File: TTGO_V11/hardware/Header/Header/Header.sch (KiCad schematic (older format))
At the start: 1 part

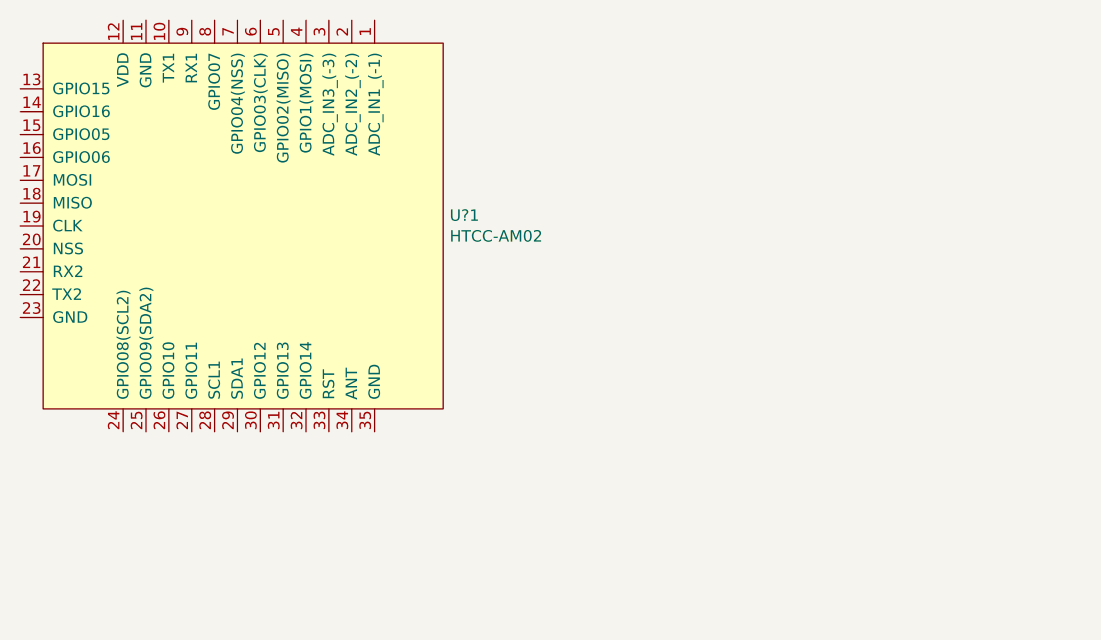
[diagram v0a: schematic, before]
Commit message: design changes
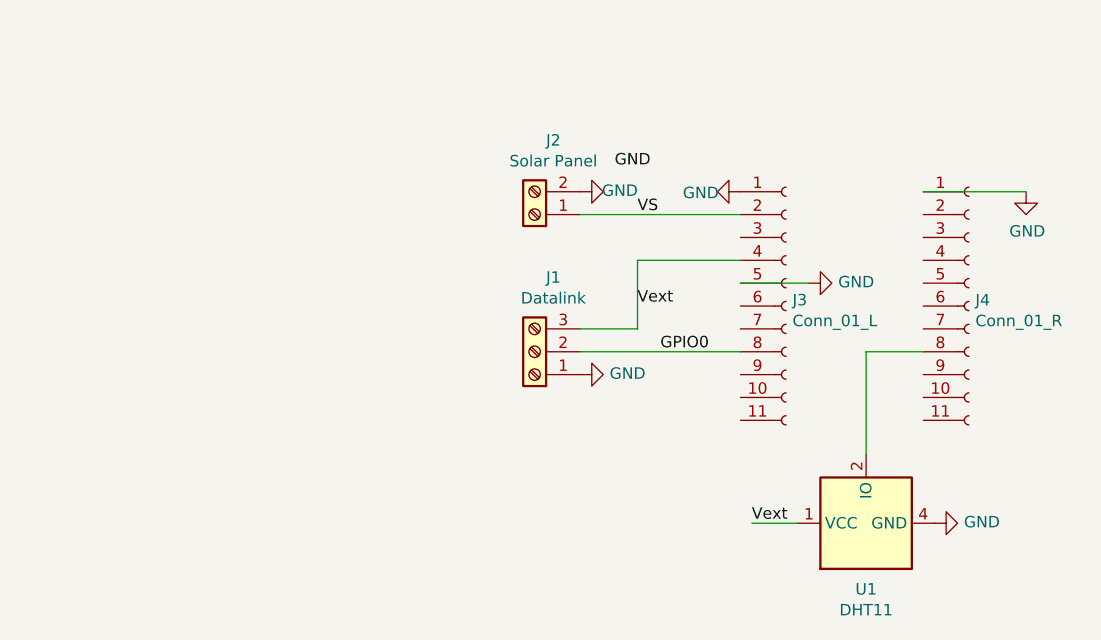
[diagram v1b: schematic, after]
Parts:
- removed U?1: HTCC-AM02, symbol htcc:HTCC-AM02
- added J1: Datalink, TerminalBlock_MetzConnect:TerminalBlock_MetzConnect_Type101_RT01603HBWC_1x03_P5.08mm_Horizontal, symbol Connector:Screw_Terminal_01x03
- added J2: Solar Panel, TerminalBlock_MetzConnect:TerminalBlock_MetzConnect_Type101_RT01602HBWC_1x02_P5.08mm_Horizontal, symbol Connector:Screw_Terminal_01x02
- added J3: Conn_01_L, Connector_PinHeader_2.54mm:PinHeader_1x11_P2.54mm_Vertical, symbol Connector:Conn_01x11_Female
- added J4: Conn_01_R, Connector_PinHeader_2.54mm:PinHeader_1x11_P2.54mm_Vertical, symbol Connector:Conn_01x11_Female
- added U1: DHT11, Sensor:Aosong_DHT11_5.5x12.0_P2.54mm, symbol Sensor:DHT11
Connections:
- new net: J4.8 (Pin_8), U1.2 (IO)
- new net GND: J1.1 (Pin_1), J2.2 (Pin_2), J3.1 (Pin_1), J3.5 (Pin_5), J4.1 (Pin_1), U1.4 (GND)
- new net GPIO0: J1.2 (Pin_2), J3.8 (Pin_8)
- new net VS: J2.1 (Pin_1), J3.2 (Pin_2)
- new net Vext: J1.3 (Pin_3), J3.4 (Pin_4), U1.1 (VCC)
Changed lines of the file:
@@
 $EndDescr
 $Comp
-L htcc:HTCC-AM02 U?1
-U 1 1 608BC1DC
-P 5750 3550
-F 0 "U?1" H 6678 3596 50  0000 L CNN
-F 1 "HTCC-AM02" H 6678 3505 50  0000 L CNN
-F 2 "" H 5800 4150 50  0001 C CNN
-F 3 "" H 5800 4150 50  0001 C CNN
-	1    5750 3550
+L Connector:Screw_Terminal_01x03 J1
+U 1 1 608CA66F
+P 7050 4100
+F 0 "J1" H 6968 3775 50  0000 C CNN
+F 1 "Datalink" H 6968 3866 50  0000 C CNN
+F 2 "TerminalBlock_MetzConnect:TerminalBlock_MetzConnect_Type101_RT01603HBWC_1x03_P5.08mm_Horizontal" H 7050 4100 50  0001 C CNN
+F 3 "~" H 7050 4100 50  0001 C CNN
+	1    7050 4100
+	-1   0    0    1
+$EndComp
+$Comp
+L Connector:Screw_Terminal_01x02 J2
+U 1 1 608CAD5D
+P 7050 3500
+F 0 "J2" H 6968 3175 50  0000 C CNN
+F 1 "Solar Panel" H 6968 3266 50  0000 C CNN
+F 2 "TerminalBlock_MetzConnect:TerminalBlock_MetzConnect_Type101_RT01602HBWC_1x02_P5.08mm_Horizontal" H 7050 3500 50  0001 C CNN
+F 3 "~" H 7050 3500 50  0001 C CNN
+	1    7050 3500
+	-1   0    0    1
+$EndComp
+$Comp
+L Connector:Conn_01x11_Female J3
+U 1 1 608CB784
+P 8150 3900
+F 0 "J3" H 8178 3926 50  0000 L CNN
+F 1 "Conn_01_L" H 8178 3835 50  0000 L CNN
+F 2 "Connector_PinHeader_2.54mm:PinHeader_1x11_P2.54mm_Vertical" H 8150 3900 50  0001 C CNN
+F 3 "~" H 8150 3900 50  0001 C CNN
+	1    8150 3900
 	1    0    0    -1
 $EndComp
+$Comp
+L Connector:Conn_01x11_Female J4
+U 1 1 608D10F0
+P 8950 3900
+F 0 "J4" H 8978 3926 50  0000 L CNN
+F 1 "Conn_01_R" H 8978 3835 50  0000 L CNN
+F 2 "Connector_PinHeader_2.54mm:PinHeader_1x11_P2.54mm_Vertical" H 8950 3900 50  0001 C CNN
+F 3 "~" H 8950 3900 50  0001 C CNN
+	1    8950 3900
+	1    0    0    -1
+$EndComp
+$Comp
+L power:GND #PWR0101
+U 1 1 608D6208
+P 7950 3400
+F 0 "#PWR0101" H 7950 3150 50  0001 C CNN
+F 1 "GND" V 7955 3227 50  0000 C CNN
+F 2 "" H 7950 3400 50  0001 C CNN
+F 3 "" H 7950 3400 50  0001 C CNN
+	1    7950 3400
+	0    1    1    0
+$EndComp
+Wire Wire Line
+	7950 3500 7250 3500
+Text Label 7500 3500 0    50   ~ 0
+VS
+Wire Wire Line
+	7950 3700 7500 3700
+Wire Wire Line
+	7500 3700 7500 4000
+Wire Wire Line
+	7500 4000 7250 4000
+Text Label 7500 3900 0    50   ~ 0
+Vext
+Wire Wire Line
+	7950 4100 7250 4100
+Text Label 7600 4100 0    50   ~ 0
+GPIO0
+$Comp
+L power:GND #PWR0102
+U 1 1 608D7AC1
+P 7250 4200
+F 0 "#PWR0102" H 7250 3950 50  0001 C CNN
+F 1 "GND" V 7255 4072 50  0000 R CNN
+F 2 "" H 7250 4200 50  0001 C CNN
+F 3 "" H 7250 4200 50  0001 C CNN
+	1    7250 4200
+	0    -1   -1   0
+$EndComp
+$Comp
+L Sensor:DHT11 U1
+U 1 1 608D9326
+P 8500 4850
+F 0 "U1" V 8211 4850 50  0000 C CNN
+F 1 "DHT11" V 8120 4850 50  0000 C CNN
+F 2 "Sensor:Aosong_DHT11_5.5x12.0_P2.54mm" H 8500 4450 50  0001 C CNN
+F 3 "http://akizukidenshi.com/download/ds/aosong/DHT11.pdf" H 8650 5100 50  0001 C CNN
+	1    8500 4850
+	0    -1   -1   0
+$EndComp
+Wire Wire Line
+	8750 4100 8500 4100
+Wire Wire Line
+	8500 4100 8500 4550
+$Comp
+L power:GND #PWR0103
+U 1 1 608DD235
+P 8800 4850
+F 0 "#PWR0103" H 8800 4600 50  0001 C CNN
+F 1 "GND" V 8805 4722 50  0000 R CNN
+F 2 "" H 8800 4850 50  0001 C CNN
+F 3 "" H 8800 4850 50  0001 C CNN
+	1    8800 4850
+	0    -1   -1   0
+$EndComp
+Wire Wire Line
+	8200 4850 8000 4850
+Text Label 8000 4850 0    50   ~ 0
+Vext
+Text Label 7400 3300 0    50   ~ 0
+GND
+$Comp
+L power:GND #PWR0104
+U 1 1 608DED0A
+P 9200 3400
+F 0 "#PWR0104" H 9200 3150 50  0001 C CNN
+F 1 "GND" H 9205 3227 50  0000 C CNN
+F 2 "" H 9200 3400 50  0001 C CNN
+F 3 "" H 9200 3400 50  0001 C CNN
+	1    9200 3400
+	1    0    0    -1
+$EndComp
+Wire Wire Line
+	9200 3400 8750 3400
+Wire Wire Line
+	8250 3800 7950 3800
+$Comp
+L power:GND #PWR0105
+U 1 1 608E322D
+P 7250 3400
+F 0 "#PWR0105" H 7250 3150 50  0001 C CNN
+F 1 "GND" V 7255 3227 50  0000 C CNN
+F 2 "" H 7250 3400 50  0001 C CNN
+F 3 "" H 7250 3400 50  0001 C CNN
+	1    7250 3400
+	0    -1   -1   0
+$EndComp
+$Comp
+L power:GND #PWR0106
+U 1 1 608E3EBC
+P 8250 3800
+F 0 "#PWR0106" H 8250 3550 50  0001 C CNN
+F 1 "GND" V 8255 3672 50  0000 R CNN
+F 2 "" H 8250 3800 50  0001 C CNN
+F 3 "" H 8250 3800 50  0001 C CNN
+	1    8250 3800
+	0    -1   -1   0
+$EndComp
 $EndSCHEMATC
